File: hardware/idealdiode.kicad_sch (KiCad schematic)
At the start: 9 parts, among them IC12 AP74502QTA8-7, Q27 NVMFWS1D7N04XMT1G, Q29 NVMFWS1D7N04XMT1G

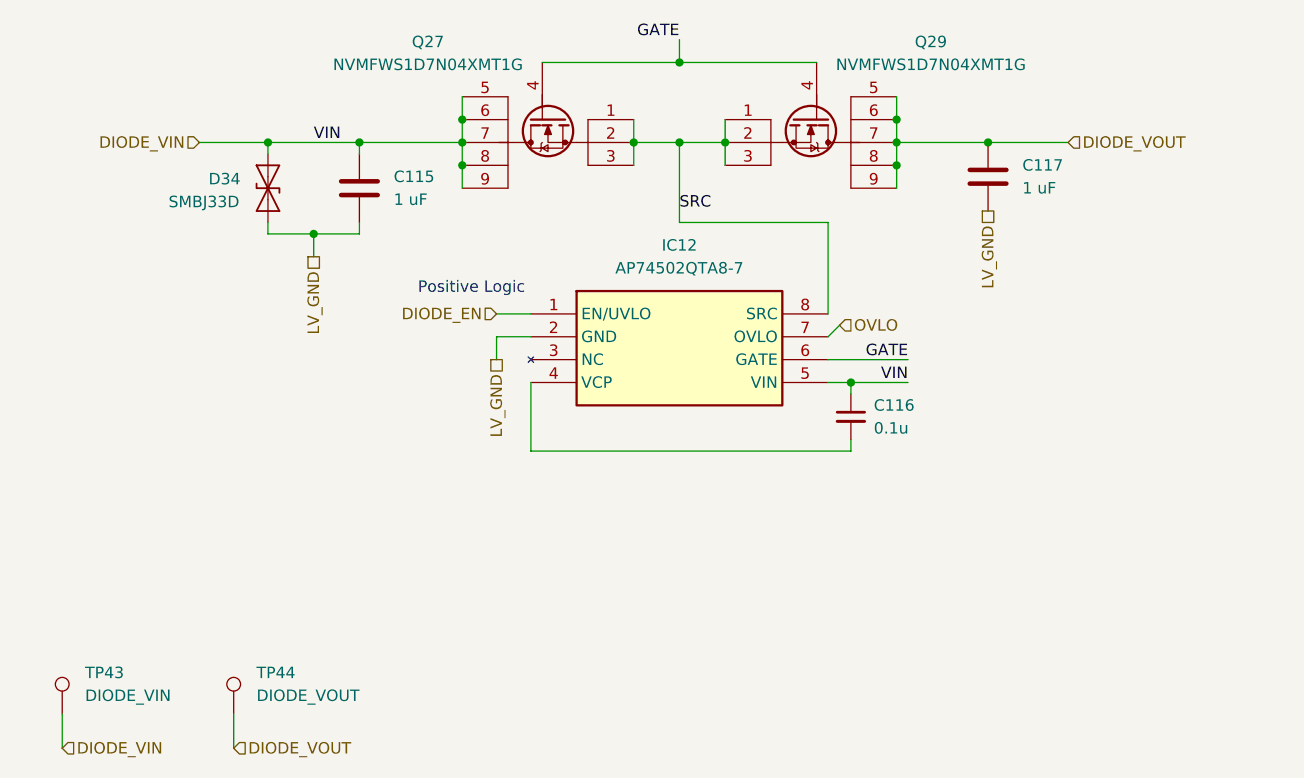
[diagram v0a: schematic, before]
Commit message: try smth on laptop
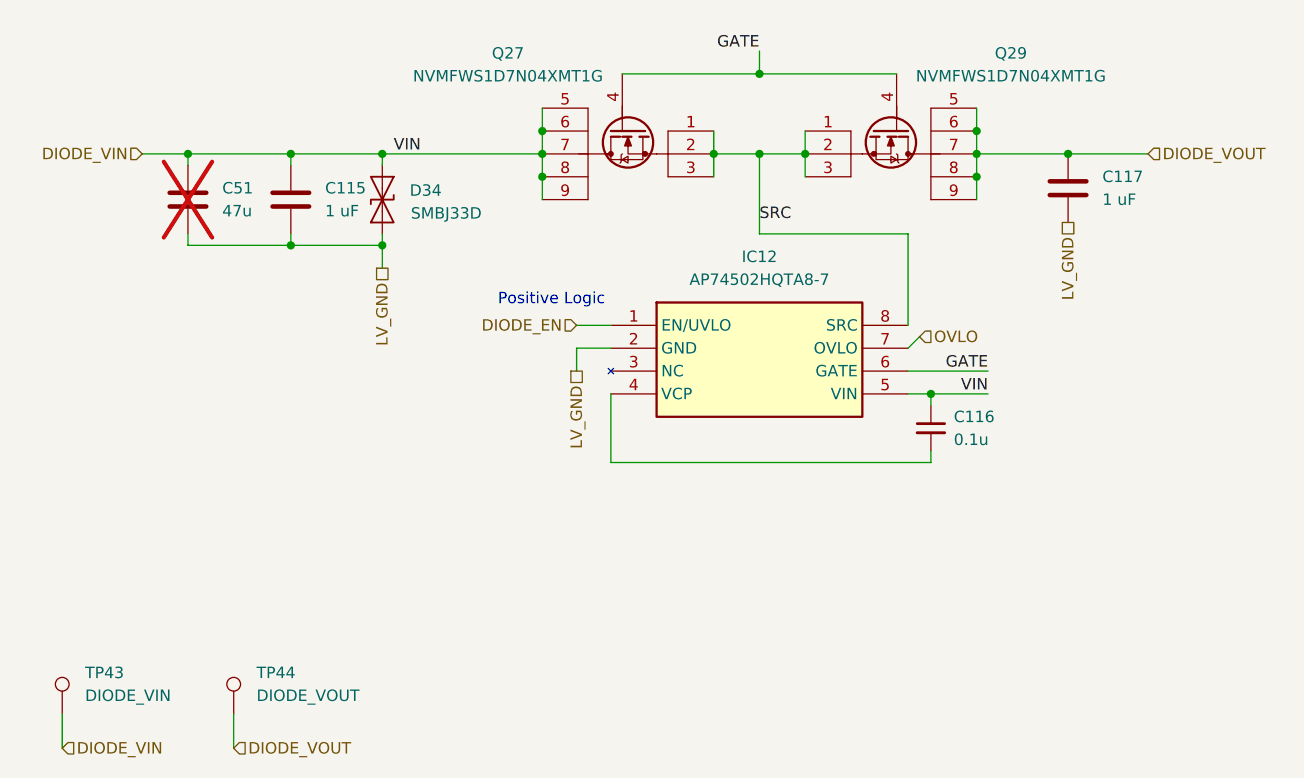
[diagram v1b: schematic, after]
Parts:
- added C51: 47u, Capacitor_SMD:C_0603_1608Metric_Pad1.08x0.95mm_HandSolder, symbol Device:C
- IC12: value AP74502QTA8-7 -> AP74502HQTA8-7
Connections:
- net DIODE_VIN: now also C51.1
- net LV_GND: now also C51.2
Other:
- moved on the sheet: C115, C116, C117, D34, IC12, Q27, Q29
